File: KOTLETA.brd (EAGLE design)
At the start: 27 x 40.2 mm, 126 parts, among them CON1 CON-6P, CON2 CON-4P-JST_GH-RA, CON3 CON-4P-JST_GH-RA, IC1 STM32F105RCT6, IC2 CAT24C02, IC3 SN65HVD232D, IC4 LMR14010ADDCT, IC5 LM75BD-TSSOP8, IC6 FAN7888, IC7 ZXCT1051, IC8 3.3V, Q1 CSD18510Q5B, Q2 CSD18510Q5B, Q3 CSD18510Q5B, Q4 CSD18510Q5B, Q5 CSD18510Q5B, Q6 CSD18510Q5B, X1 24MHz

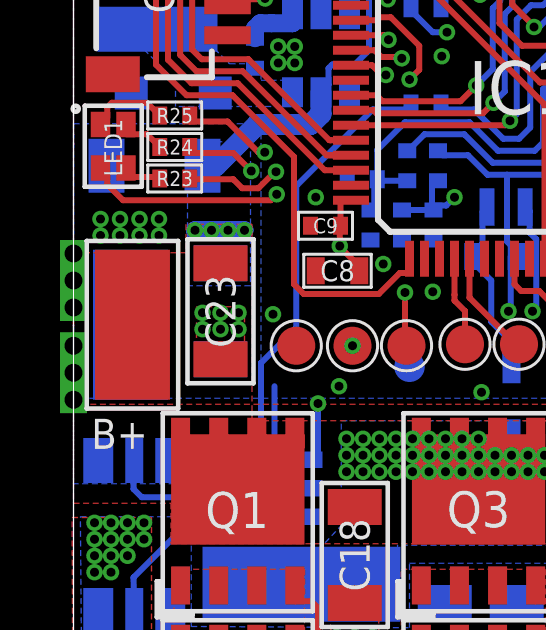
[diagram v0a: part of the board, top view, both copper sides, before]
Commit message: BOM updates
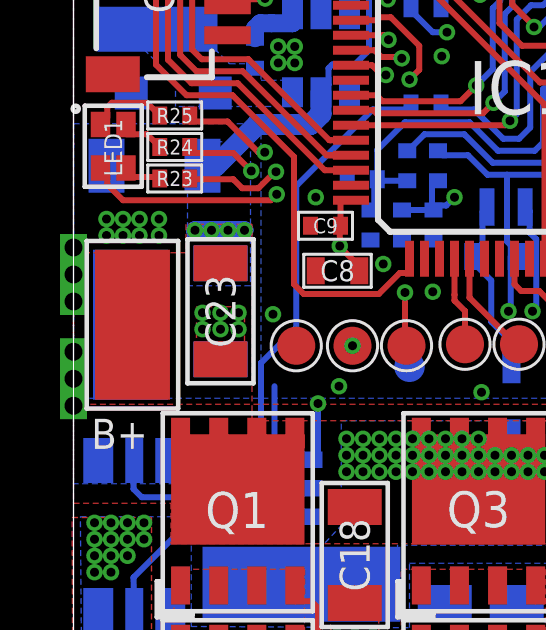
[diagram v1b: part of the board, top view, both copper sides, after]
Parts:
- C24, C30, C32: value 2.2nF -> 1800pF
- R13, R18, R22: value 3K9 -> 4K7
- moved PAD3 0.20 mm to (0.00, 18.7)
- moved PAD5 0.20 mm to (0.00, 16.1)
- moved PAD1 0.20 mm to (0.00, 20.5)
- moved PAD2 0.20 mm to (0.00, 19.6)
- moved PAD4 0.20 mm to (0.00, 15.2)
- moved PAD6 0.20 mm to (0.00, 17.1)
